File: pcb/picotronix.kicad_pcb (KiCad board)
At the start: 2 copper layers, 88.5 x 67 mm, 27 parts, among them J1 Conn_02x04_Odd_Even, J2 Conn_02x04_Odd_Even, J3 DEBUG, J4 DB25_Male, U1 Pico, U2 LSF0204DPWR, U3 AD5663R, U4 ADA4891-3

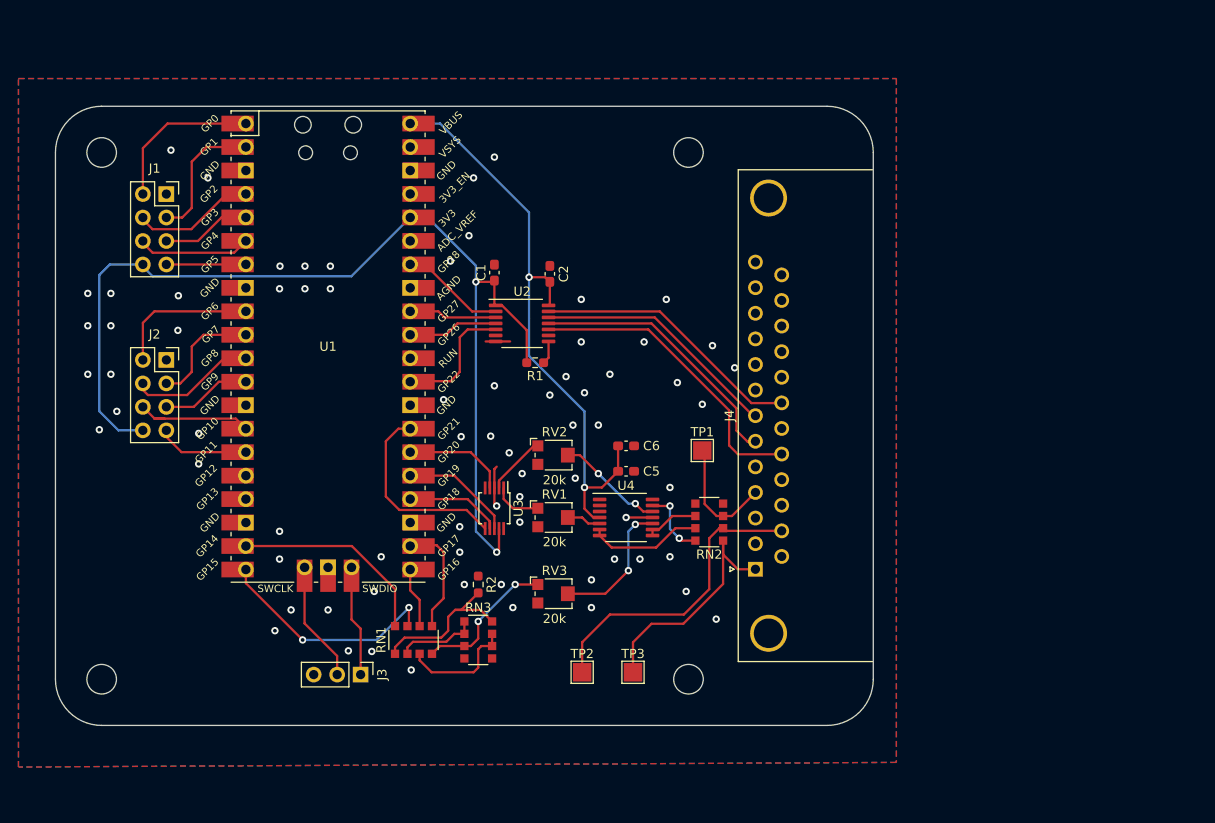
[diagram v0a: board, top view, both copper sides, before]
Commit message: pcb rev2 routed
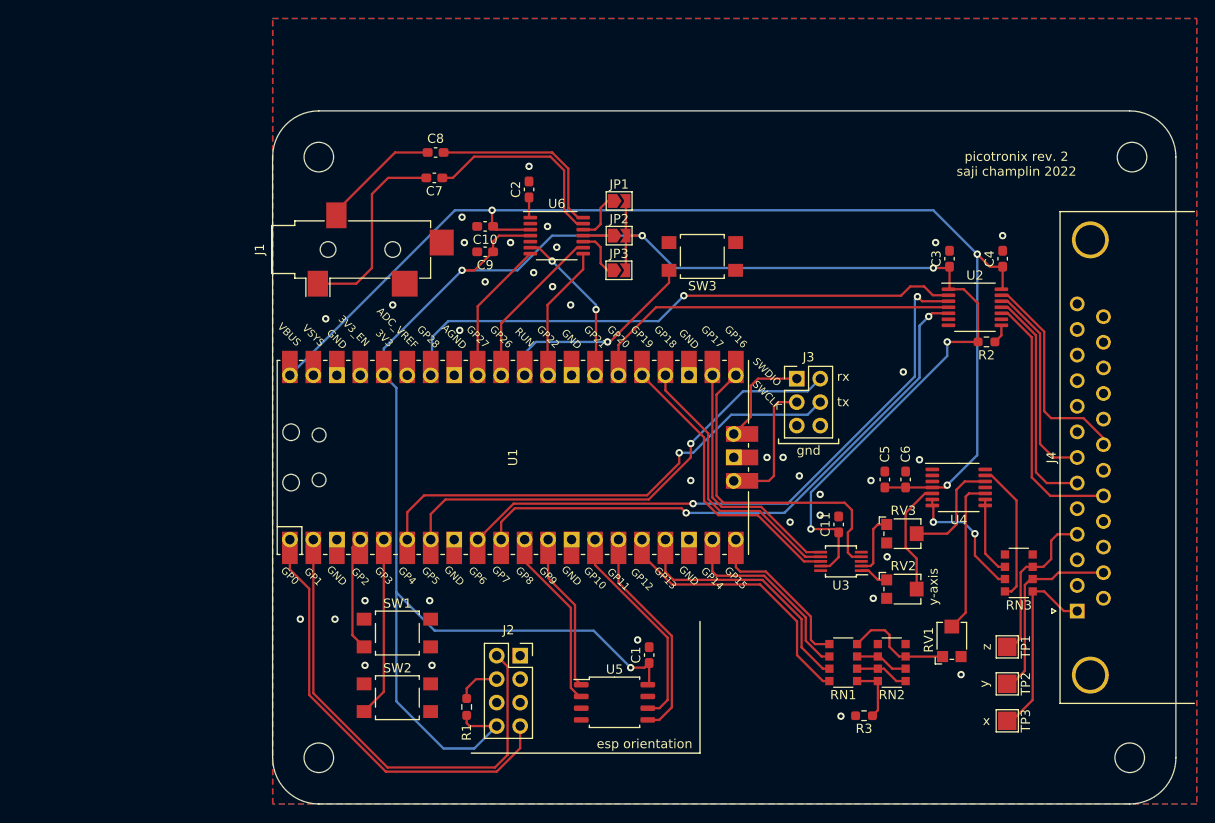
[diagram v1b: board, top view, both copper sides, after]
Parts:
- added C10: 0.1u, Capacitor_SMD:C_0603_1608Metric_Pad1.08x0.95mm_HandSolder, F.Cu at (109.0, 77.5)
- added C11: 0.1u, Capacitor_SMD:C_0603_1608Metric_Pad1.08x0.95mm_HandSolder, F.Cu at (147.2, 109.8)
- added C3: 0.1u, Capacitor_SMD:C_0603_1608Metric_Pad1.08x0.95mm_HandSolder, F.Cu at (159.2, 81.0)
- added C4: 0.1u, Capacitor_SMD:C_0603_1608Metric_Pad1.08x0.95mm_HandSolder, F.Cu at (165.0, 81.0)
- added C7: 1u, Capacitor_SMD:C_0603_1608Metric_Pad1.08x0.95mm_HandSolder, F.Cu at (103.5, 72.2)
- added C8: 1u, Capacitor_SMD:C_0603_1608Metric_Pad1.08x0.95mm_HandSolder, F.Cu at (103.6, 69.5)
- added C9: 0.1u, Capacitor_SMD:C_0603_1608Metric_Pad1.08x0.95mm_HandSolder, F.Cu at (109.0, 80.2)
- added JP1: FMT_SET, Jumper:SolderJumper-2_P1.3mm_Open_TrianglePad1.0x1.5mm, F.Cu at (123.5, 74.8)
- added JP2: MD1_SET, Jumper:SolderJumper-2_P1.3mm_Open_TrianglePad1.0x1.5mm, F.Cu at (123.5, 78.5)
- added JP3: MD0_SET, Jumper:SolderJumper-2_P1.3mm_Open_TrianglePad1.0x1.5mm, F.Cu at (123.5, 82.2)
- added R3: 10k, Resistor_SMD:R_0603_1608Metric_Pad0.98x0.95mm_HandSolder, F.Cu at (150.0, 130.4)
- added SW1: BTN0, Button_Switch_SMD:SW_SPST_TL3305A, F.Cu at (99.5, 121.5)
- added SW2: BTN1, Button_Switch_SMD:SW_SPST_TL3305A, F.Cu at (99.5, 128.5)
- added SW3: RESET, Button_Switch_SMD:SW_SPST_TL3305A, F.Cu at (132.5, 80.8)
- added U5: W25Q128JVS, Package_SO:SOIC-8_5.23x5.23mm_P1.27mm, F.Cu at (123.0, 129.0)
- added U6: PCM1808, Package_SO:TSSOP-14_4.4x5mm_P0.65mm, F.Cu at (116.8, 78.5)
- J1: value Conn_02x04_Odd_Even -> AudioJack3_Ground; footprint Connector_PinSocket_2.54mm:PinSocket_2x04_P2.54mm_Vertical -> Connector_Audio:Jack_3.5mm_CUI_SJ-3524-SMT_Horizontal
- J2: value Conn_02x04_Odd_Even -> ESP-01 Connector
- J3: footprint Connector_PinHeader_2.54mm:PinHeader_1x03_P2.54mm_Vertical -> Connector_PinHeader_2.54mm:PinHeader_2x03_P2.54mm_Vertical
- RN2: value 470 -> 4.99k
- RN3: value 4.99k -> 470
- moved R2 60.9 mm to (163.2, 90.0), turned to 180 degrees
- moved RN3 58.9 mm to (166.8, 115.0), turned to 180 degrees
- moved J3 57.0 mm to (142.7, 94.0), turned to 0 degrees
- moved J2 49.9 mm to (112.8, 124.0)
- moved U2 49.0 mm to (162.0, 86.2)
- moved H4 48.5 mm to (178.8, 135.0)
- moved H2 48.0 mm to (179.0, 70.0)
- moved RN1 46.6 mm to (147.8, 124.7), turned to 180 degrees
- moved TP2 46.0 mm to (165.5, 127.0), turned to -90 degrees
- moved RV1 45.0 mm to (159.5, 122.2), turned to 90 degrees
- moved C1 44.6 mm to (126.8, 123.9)
- moved TP3 40.8 mm to (165.5, 131.0), turned to -90 degrees
- moved RV2 40.4 mm to (154.2, 116.8)
- moved TP1 39.2 mm to (165.5, 123.0), turned to -90 degrees
- moved RV3 38.3 mm to (154.2, 110.8)
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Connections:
- C2 pad 1: +5V -> Net-(C2-Pad1)
- J2 pad 2: /gpio6 -> /UART0_RX
- J2 pad 3: /gpio7 -> unconnected-(J2-Pad3)
- J2 pad 4: /gpio8 -> /esp_en
- J2 pad 5: /gpio9 -> unconnected-(J2-Pad5)
- J2 pad 6: /gpio10 -> unconnected-(J2-Pad6)
- J2 pad 7: /gpio11 -> /UART0_TX
- J3 pad 2: Net-(J3-Pad2) -> /dbg_rx
- J3 pad 3: GND -> Net-(J3-Pad3)
- R1 pad 1: Net-(R1-Pad1) -> +3V3
- R1 pad 2: +3V3 -> /esp_en
- R2 pad 1: GND -> Net-(R2-Pad1)
- R2 pad 2: Net-(R2-Pad2) -> +3V3
- RN1 pad 1: Net-(R2-Pad2) -> Net-(R3-Pad2)
- RN2 pad 1: /X_OUTPUT -> Net-(RN1-Pad2)
- RN2 pad 2: /Y_OUTPUT -> Net-(RN1-Pad3)
- RN2 pad 3: /Z_OUTPUT -> Net-(RN1-Pad4)
- RN2 pad 6: Net-(RN2-Pad6) -> Net-(RN1-Pad3)
- RN2 pad 7: Net-(RN2-Pad7) -> Net-(RN1-Pad2)
- RN2 pad 8: Net-(RN2-Pad8) -> Net-(R3-Pad2)
- RN3 pad 1: Net-(RN1-Pad2) -> /X_OUTPUT
- RN3 pad 2: Net-(RN1-Pad2) -> /Y_OUTPUT
- RN3 pad 3: Net-(RN1-Pad4) -> /Z_OUTPUT
- RN3 pad 6: Net-(RN1-Pad3) -> Net-(RN3-Pad6)
- RN3 pad 7: Net-(RN1-Pad3) -> Net-(RN3-Pad7)
- RN3 pad 8: Net-(R2-Pad2) -> Net-(RN3-Pad8)
- RV1 pad 1: Net-(RV1-Pad1) -> Net-(RN1-Pad4)
- RV3 pad 1: Net-(RN1-Pad4) -> Net-(RV3-Pad1)
- U1 pad 1: /gpio0 -> /UART0_TX
- U1 pad 10: /gpio7 -> /erase_l
- U1 pad 11: /gpio8 -> /FLASH_MISO
- U1 pad 12: /gpio9 -> /FLASH_CS
- U1 pad 14: /gpio10 -> /FLASH_SCK
- U1 pad 15: /gpio11 -> /FLASH_MOSI
- U1 pad 16: unconnected-(U1-Pad16) -> /z_{1}
- U1 pad 17: unconnected-(U1-Pad17) -> /z_{2}
- U1 pad 19: /z_{1} -> /z_{3}
- U1 pad 2: /gpio1 -> /UART0_RX
- U1 pad 20: /z_{2} -> /z_{4}
- U1 pad 21: /z_{3} -> /XY_FLUSH
- U1 pad 22: /z_{4} -> /~{CS}
- U1 pad 26: /XY_FLUSH -> /non_store_l
- U1 pad 27: /~{CS} -> /i2s_mclk
- U1 pad 29: /erase_l -> /i2s_bck
- U1 pad 30: unconnected-(U1-Pad30) -> Net-(SW3-Pad1)
- U1 pad 31: /non_store_l -> /i2s_dout
- U1 pad 32: /erase_interval_l -> /i2s_lrclk
- U1 pad 4: /gpio2 -> Net-(SW1-Pad2)
- U1 pad 41: Net-(J3-Pad2) -> Net-(J3-Pad3)
- U1 pad 5: /gpio3 -> Net-(SW2-Pad2)
- U1 pad 6: /gpio4 -> /dbg_tx
- U1 pad 7: /gpio5 -> /dbg_rx
- U1 pad 9: /gpio6 -> /erase_interval_l
- U2 pad 8: Net-(R1-Pad1) -> Net-(R2-Pad1)
- U3 pad 1: Net-(RV1-Pad1) -> Net-(RV2-Pad1)
- U3 pad 2: Net-(RV2-Pad1) -> Net-(RV3-Pad1)
- U4 pad 10: Net-(RV3-Pad2) -> Net-(RV1-Pad2)
- U4 pad 12: Net-(RV2-Pad2) -> Net-(RV3-Pad2)
- U4 pad 13: Net-(RN2-Pad8) -> Net-(RN3-Pad8)
- U4 pad 5: Net-(RV1-Pad2) -> Net-(RV2-Pad2)
- U4 pad 6: Net-(RN2-Pad7) -> Net-(RN3-Pad7)
- U4 pad 7: Net-(RN2-Pad7) -> Net-(RN3-Pad7)
- U4 pad 8: Net-(RN2-Pad6) -> Net-(RN3-Pad6)
- U4 pad 9: Net-(RN2-Pad6) -> Net-(RN3-Pad6)
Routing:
- net +3V3: track 113.5 -> 224.9 mm, vias 2 -> 6
- net +5V: track 65.6 -> 128.6 mm, vias 2 -> 3
- net /erase_interval_l: track 9.52 -> 66.9 mm, vias 0 -> 2
- net /dbg_tx: track 0.00 -> 53.2 mm, vias 0 -> 1
- net /UART0_RX: track 0.00 -> 52.8 mm
- net /dbg_rx: track 0.00 -> 51.9 mm, vias 0 -> 1
- net /var_bright_l: track 11.4 -> 62.5 mm, vias 0 -> 1
- net /erase_l: track 13.8 -> 63.4 mm, vias 0 -> 2
- net /UART0_TX: track 0.00 -> 47.4 mm
- net /non_store_l: track 9.76 -> 40.7 mm
- net /XY_FLUSH: track 11.3 -> 35.6 mm
- net /FLASH_MOSI: track 0.00 -> 23.7 mm
- net /FLASH_SCK: track 0.00 -> 23.1 mm
- net Net-(SW3-Pad1): track 0.00 -> 22.5 mm, vias 0 -> 1
- net Net-(C7-Pad1): track 0.00 -> 21.8 mm
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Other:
- board size 88.5 x 67 mm -> 97.8 x 75 mm
- board text added: "SWCLK"
- board text added: "SWDIO"
- board text added: "esp orientation"
- board text added: "gnd"
- board text added: "picotronix rev. 2 saji champlin 2022"
- board text added: "rx"
- board text added: "tx"
- board text added: "x"
- board text added: "y"
- board text added: "y-axis"
- board text added: "z"
- board text removed: "picotronix rev.1 saji champlin 03/2022"
